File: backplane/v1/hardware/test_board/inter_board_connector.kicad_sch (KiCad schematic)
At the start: 1 part, among them J1 Conn_02x20_Odd_Even

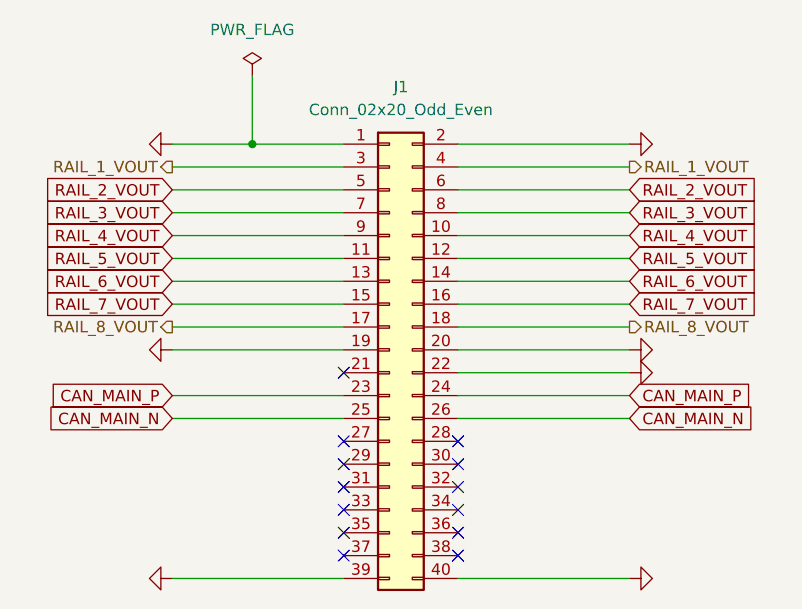
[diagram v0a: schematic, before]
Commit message: start layout
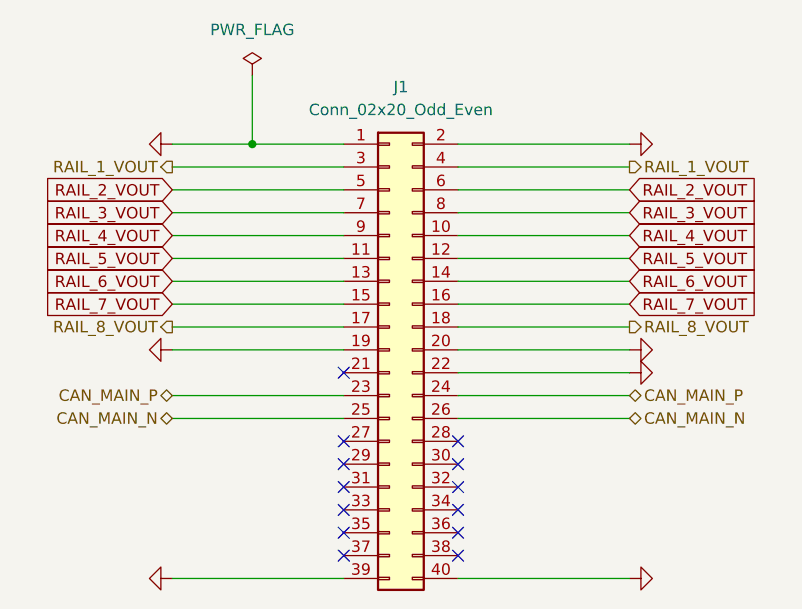
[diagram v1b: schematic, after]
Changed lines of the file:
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@@
-		)
-	)
-	(global_label "CAN_MAIN_N"
-		(shape input)
-		(at 152.4 100.33 0)
-		(fields_autoplaced yes)
-		(effects
-			(font
-				(size 1.27 1.27)
-			)
-			(justify left)
-		)
-		(property "Intersheetrefs" "${INTERSHEET_REFS}"
-			(at 166.5129 100.33 0)
-			(hide yes)
-			(show_name no)
-			(do_not_autoplace no)
-			(effects
-				(font
-					(size 1.27 1.27)
-				)
-				(justify left)
-			)
 		)
 	)
@@
 		)
 	)
-	(global_label "CAN_MAIN_P"
-		(shape input)
-		(at 152.4 97.79 0)
-		(fields_autoplaced yes)
-		(effects
-			(font
-				(size 1.27 1.27)
-			)
-			(justify left)
-		)
-		(property "Intersheetrefs" "${INTERSHEET_REFS}"
-			(at 166.8153 97.79 0)
-			(hide yes)
-			(show_name no)
-			(do_not_autoplace no)
-			(effects
-				(font
-					(size 1.27 1.27)
-				)
-				(justify left)
-			)
-		)
-	)
 	(global_label "RAIL_7_VOUT"
 		(shape input)
@@
 		)
 	)
-	(global_label "CAN_MAIN_N"
-		(shape input)
-		(at 101.6 100.33 180)
-		(fields_autoplaced yes)
-		(effects
-			(font
-				(size 1.27 1.27)
-			)
-			(justify right)
-		)
-		(property "Intersheetrefs" "${INTERSHEET_REFS}"
-			(at 87.1847 100.33 0)
-			(hide yes)
-			(show_name no)
-			(do_not_autoplace no)
-			(effects
-				(font
-					(size 1.27 1.27)
-				)
-				(justify right)
-			)
-		)
-	)
 	(global_label "RAIL_2_VOUT"
 		(shape input)
@@
 		(property "Intersheetrefs" "${INTERSHEET_REFS}"
 			(at 86.7614 74.93 0)
-			(hide yes)
-			(show_name no)
-			(do_not_autoplace no)
-			(effects
-				(font
-					(size 1.27 1.27)
-				)
-				(justify right)
-			)
-		)
-	)
-	(global_label "CAN_MAIN_P"
-		(shape input)
-		(at 101.6 97.79 180)
-		(fields_autoplaced yes)
-		(effects
-			(font
-				(size 1.27 1.27)
-			)
-			(justify right)
-		)
-		(property "Intersheetrefs" "${INTERSHEET_REFS}"
-			(at 87.2452 97.79 0)
 			(hide yes)
 			(show_name no)
@@
 		)
 	)
+	(hierarchical_label "CAN_MAIN_N"
+		(shape bidirectional)
+		(at 152.4 100.33 0)
+		(effects
+			(font
+				(size 1.27 1.27)
+			)
+			(justify left)
+		)
+	)
 	(hierarchical_label "RAIL_1_VOUT"
 		(shape output)
@@
 			)
 			(justify left)
+		)
+	)
+	(hierarchical_label "CAN_MAIN_P"
+		(shape bidirectional)
+		(at 101.6 97.79 180)
+		(effects
+			(font
+				(size 1.27 1.27)
+			)
+			(justify right)
+		)
+	)
+	(hierarchical_label "CAN_MAIN_N"
+		(shape bidirectional)
+		(at 101.6 100.33 180)
+		(effects
+			(font
+				(size 1.27 1.27)
+			)
+			(justify right)
+		)
+	)
+	(hierarchical_label "CAN_MAIN_P"
+		(shape bidirectional)
+		(at 152.4 97.79 0)
+		(effects
+			(font
+				(size 1.27 1.27)
+			)
+			(justify left)
